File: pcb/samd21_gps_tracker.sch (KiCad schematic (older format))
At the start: 94 parts, among them J1 JTAG_SWD_6, J2 01x04, J3 U.FL-R-SMT, J4 SIM_Card, J5 USB_C_Receptacle_USB2.0, J6 U.FL-R-SMT, Q1 2N7002, Q2 2N7002, Q3 2N7002, Q4 2N7002, Q5 2N7002, Q6 Q_PMOS_GSD, Q7 Q_PMOS_GSD, Q8 Q_PMOS_GSD, Q9 2N7002, SW1 SW_Push, SW2 SW_Push_SPDT, U1 XL1509_SOP8, U2 ATSAMD21G18A-A, U3 MCP2515-xSO, U4 L96-M33, U5 RN2903, U6 MCP2551-I-SN, U7 LIS2DE12, U8 SIM7020E, U9 ME6208, Y1 32.768k, Y2 16mHz

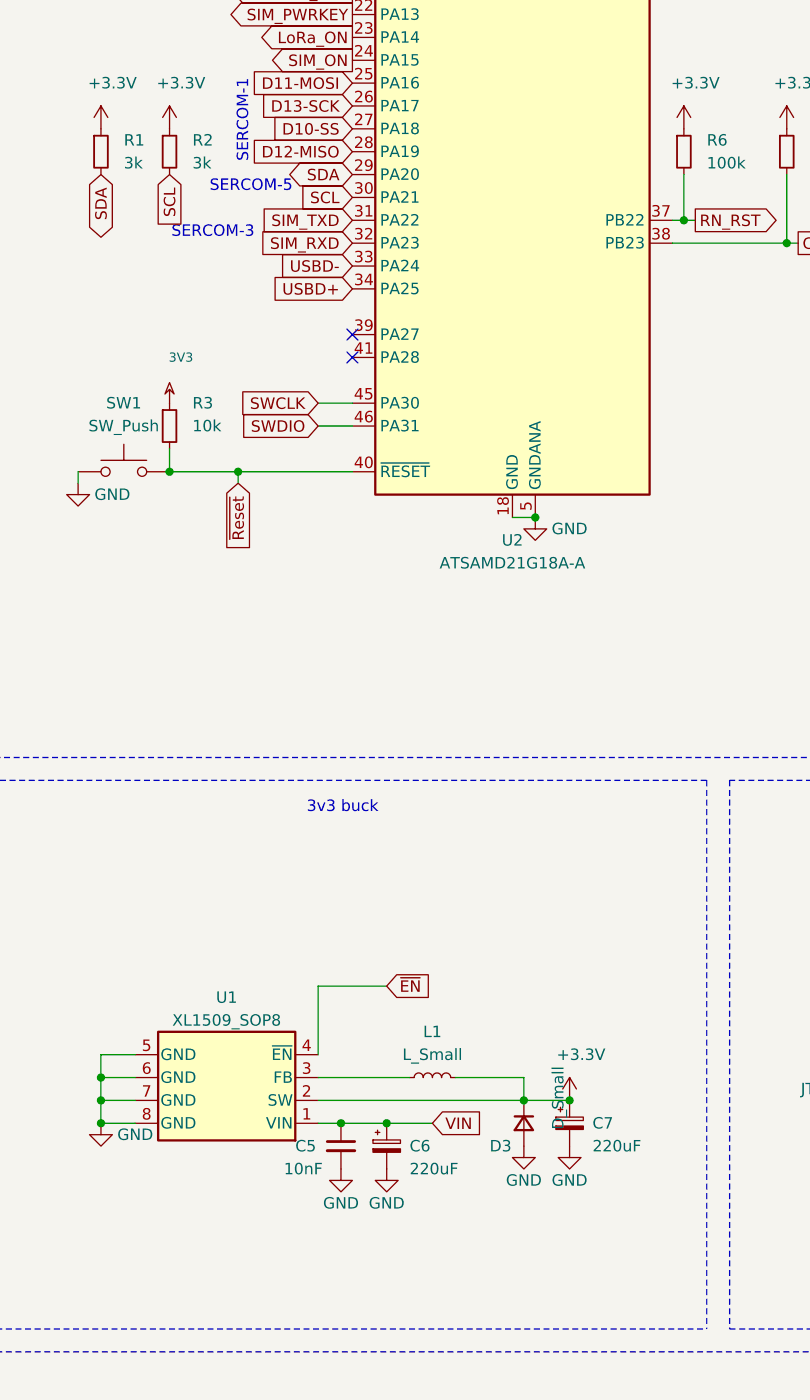
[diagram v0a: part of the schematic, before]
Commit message: WIP
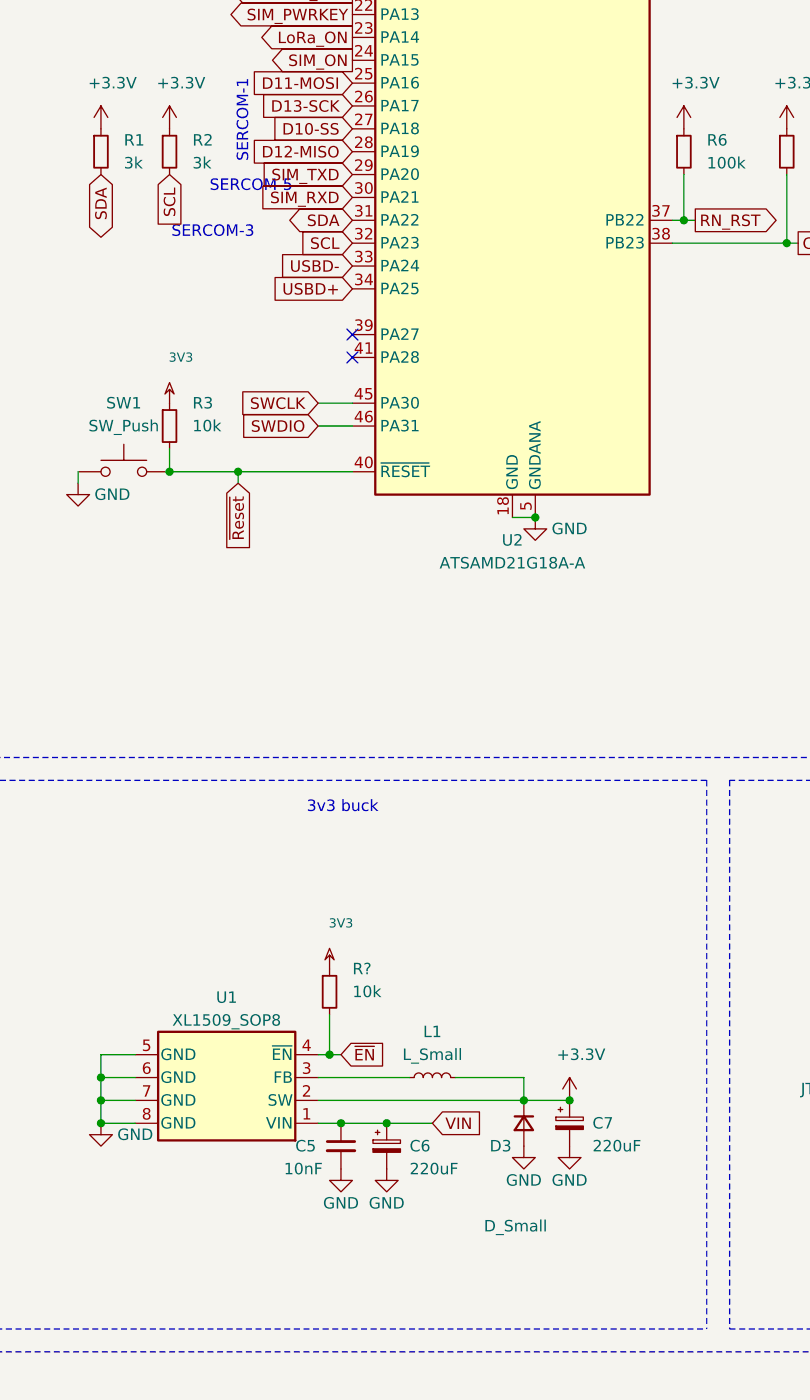
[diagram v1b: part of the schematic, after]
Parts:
- added R?: 10k, Resistor_SMD:R_0603_1608Metric, symbol Device:R_Small
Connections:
- net 3V3: now also R?.1
- net SCL: now also U2.32 (PA23); no longer U2.30 (PA21)
- net SDA: now also U2.31 (PA22); no longer U2.29 (PA20)
- net SIM_RXD: now also U2.30 (PA21); no longer U2.32 (PA23)
- net SIM_TXD: now also U2.29 (PA20); no longer U2.31 (PA22)
- net ~EN: now also R?.2
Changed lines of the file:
@@
 Text GLabel 2100 3700 0    50   Output ~ 0
 STATUS_LED
-Text GLabel 2100 4500 0    50   BiDi ~ 0
+Text GLabel 2100 4700 0    50   BiDi ~ 0
 SDA
-Text GLabel 2100 4600 0    50   Input ~ 0
+Text GLabel 2100 4800 0    50   Input ~ 0
 SCL
 Text GLabel 2100 4900 0    50   Input ~ 0
@@
 P 2850 8650
 F 0 "D3" V 2950 8500 50  0000 L CNN
-F 1 "D_Small" H 2600 8800 50  0000 L CNN
+F 1 "D_Small" V 3300 8475 50  0000 L CNN
 F 2 "Diode_SMD:D_SMA" V 2850 8650 50  0001 C CNN
 F 3 "~" V 2850 8650 50  0001 C CNN
@@
 Wire Wire Line
 	11250 1600 11350 1600
-Text GLabel 2250 8050 2    50   Input ~ 0
+Text GLabel 2050 8350 2    50   Input ~ 0
 ~EN
 Text GLabel 5650 1200 2    50   Input ~ 0
@@
 SIM_PWRKEY
 NoConn ~ 13350 5650
-Text GLabel 2100 4800 0    50   Input ~ 0
+Text GLabel 2100 4600 0    50   Input ~ 0
 SIM_RXD
-Text GLabel 2100 4700 0    50   Input ~ 0
+Text GLabel 2100 4500 0    50   Input ~ 0
 SIM_TXD
 NoConn ~ 7550 5300
@@
 Text Notes 9600 8400 0    50   ~ 0
 Unfuck the CAN tranceiver you tard. Needs to be 3.3v
-Wire Wire Line
-	1950 8350 1950 8050
 Text Notes 8400 10200 0    50   ~ 0
 C7244 - Plug
 Wire Wire Line
-	1950 8050 2250 8050
-Wire Wire Line
 	7000 1100 7000 1000
 Wire Wire Line
@@
 Wire Wire Line
 	9400 4750 9550 4750
+$Comp
+L Device:R_Small R?
+U 1 1 61627045
+P 2000 8075
+F 0 "R?" H 2100 8175 50  0000 L CNN
+F 1 "10k" H 2100 8075 50  0000 L CNN
+F 2 "Resistor_SMD:R_0603_1608Metric" H 2000 8075 50  0001 C CNN
+F 3 "~" H 2000 8075 50  0001 C CNN
+F 4 "C25804" H 2000 8075 50  0001 C CNN "lcsc_part_number"
+	1    2000 8075
+	1    0    0    -1
+$EndComp
+$Comp
+L MAX17260:3V3 #PWR?
+U 1 1 6162704B
+P 2000 7975
+F 0 "#PWR?" H 2000 8075 40  0001 C CNN
+F 1 "3V3" H 2050 8175 40  0000 C CNN
+F 2 "" H 2000 7975 60  0000 C CNN
+F 3 "" H 2000 7975 60  0000 C CNN
+	1    2000 7975
+	1    0    0    -1
+$EndComp
+Wire Wire Line
+	1950 8350 2000 8350
+Wire Wire Line
+	2000 8350 2000 8175
+Wire Wire Line
+	2050 8350 2000 8350
+Connection ~ 2000 8350
 $EndSCHEMATC
